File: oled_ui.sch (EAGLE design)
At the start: 30 parts

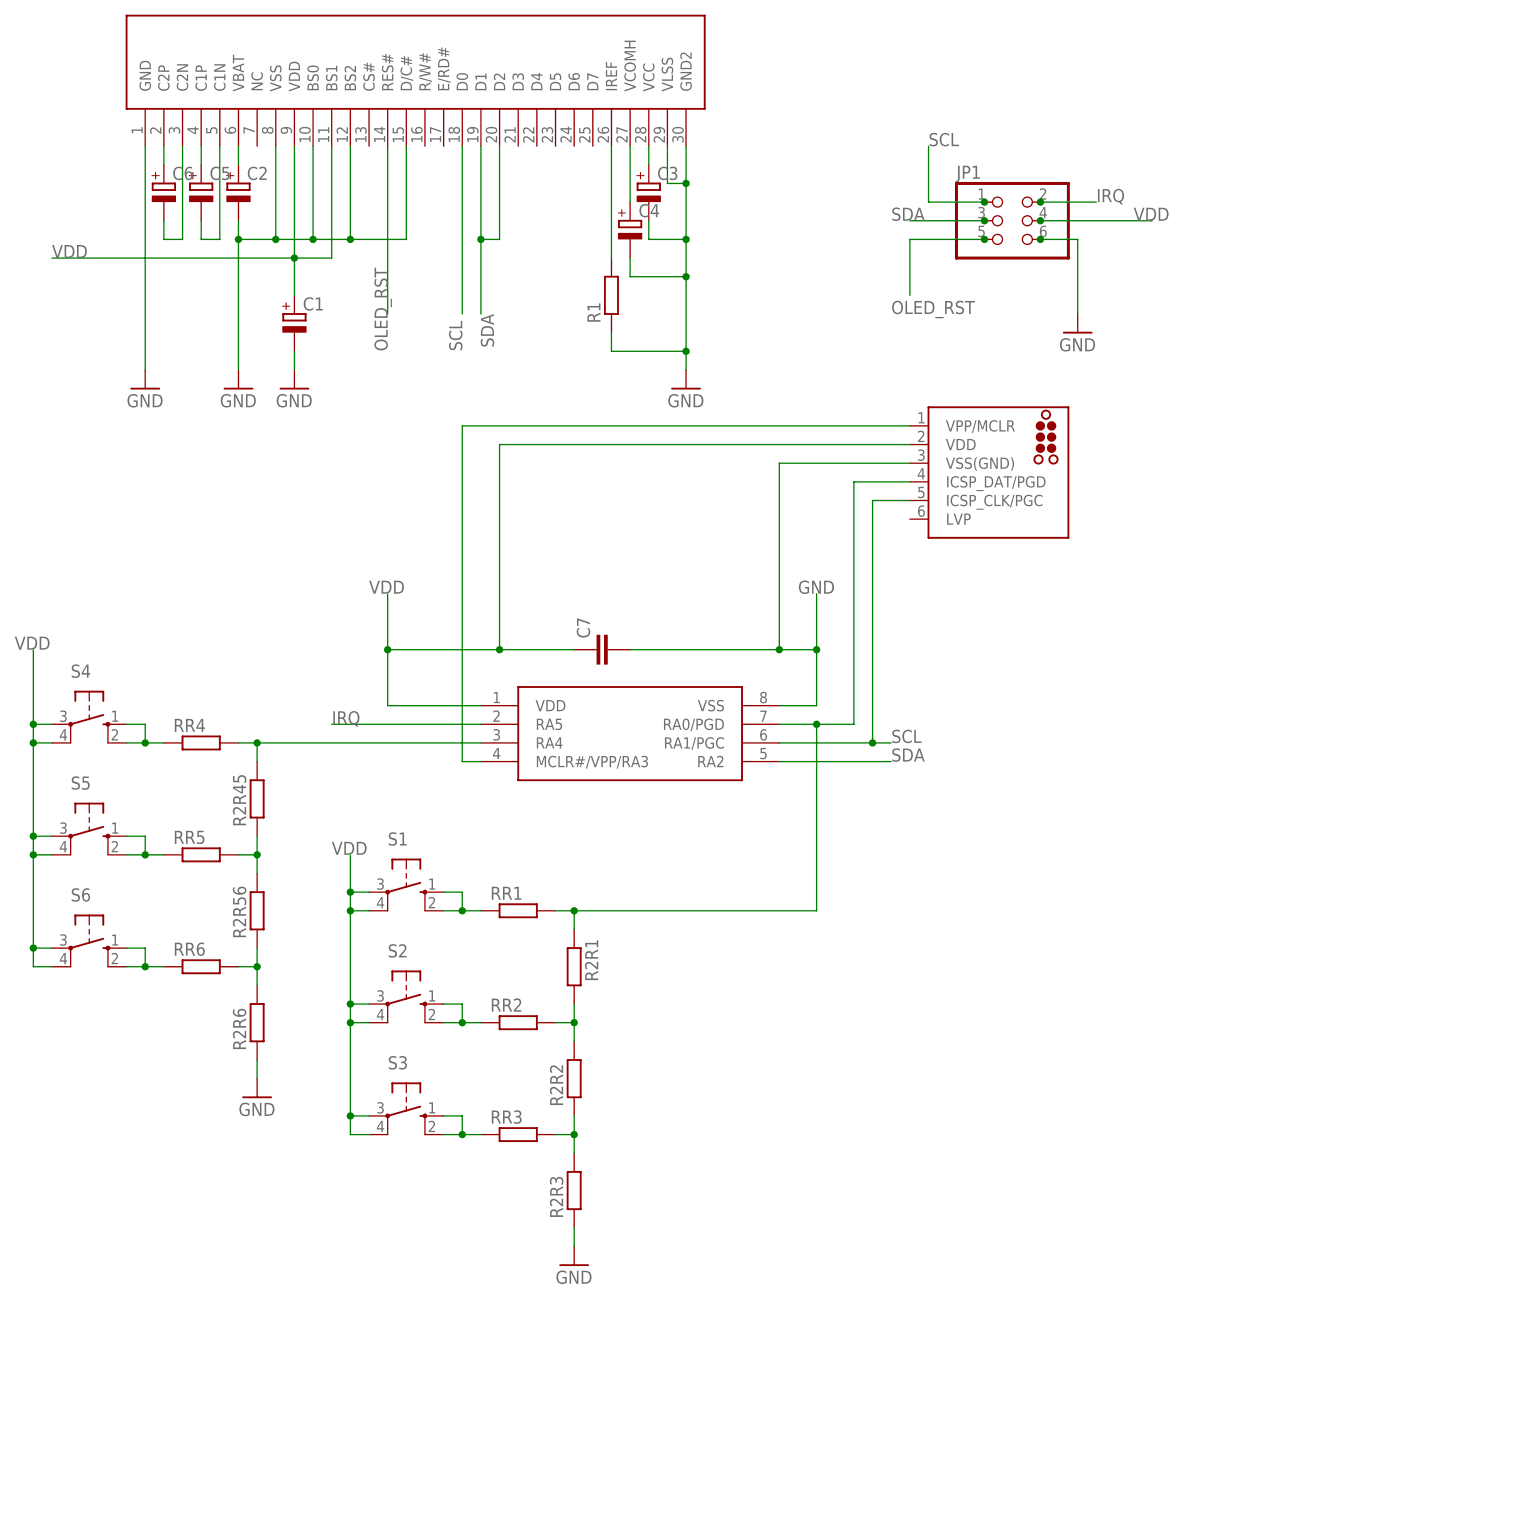
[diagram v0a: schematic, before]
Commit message: updates
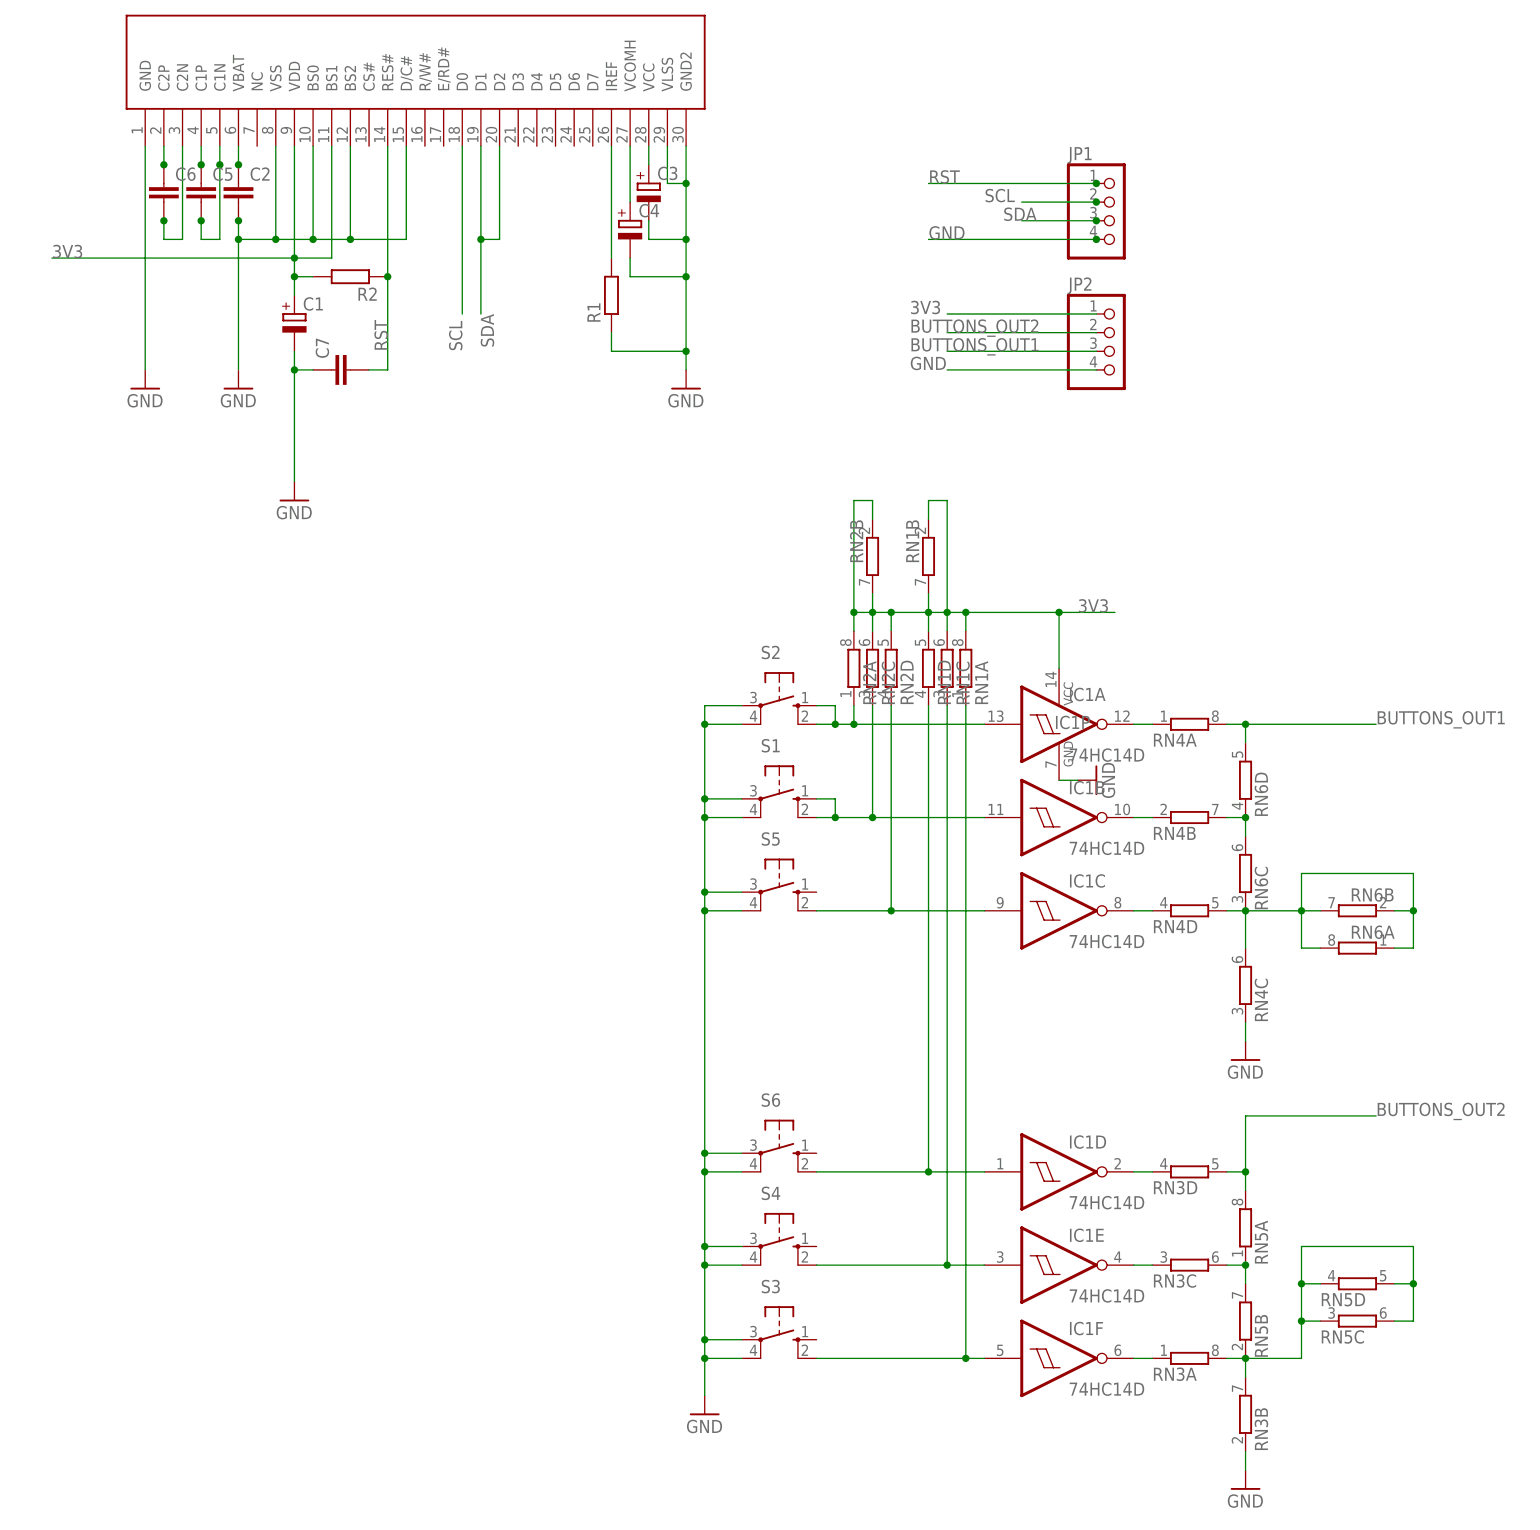
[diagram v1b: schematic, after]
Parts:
- removed J1: (no value), tag-connect:TC2030-MCP-NL
- removed R2R1, R2R2, R2R3, R2R45, R2R56, R2R6, RR1, RR2, RR3, RR4, RR5, RR6: (no value), rcl:R-EU_R0805
- removed U$2: PIC12F1822SO08, jasons_stuff:PIC12F1822SO08
- added IC1: 74HC14D, 74xx-eu:74HC14D
- added JP2: (no value), pinhead:PINHD-1X4
- added R2: (no value), rcl:R-EU_R0805
- added RN1, RN2, RN3, RN4, RN5, RN6: (no value), resistor-dil:4R-NCAY16
- C2, C5, C6: device resistor:CPOL-EUSMCA -> rcl:C-EUC0805
- JP1: device pinhead:PINHD-2X3 -> pinhead:PINHD-1X4
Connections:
- removed net IRQ: JP1.2, U$2.RA5
- removed net OLED_RST: JP1.5, U$1.RES#
- removed net VDD: C1.+, C7.1, J1.VDD, JP1.4, S1.P, S1.P1, S2.P, S2.P1, S3.P, S3.P1, S4.P, S4.P1, S5.P, S5.P1, S6.P, S6.P1, U$1.BS1, U$1.VDD, U$2.VDD
- new net 3V3: C1.+, IC1P.VCC, JP2.1, R2.2, RN1A.2, RN1B.1, RN1B.2, RN1C.2, RN1D.2, RN2A.2, RN2B.1, RN2B.2, RN2C.2, RN2D.2, U$1.BS1, U$1.VDD
- new net BUTTONS_OUT1: JP2.3, RN4A.2, RN6D.2
- new net BUTTONS_OUT2: JP2.2, RN3D.2, RN5A.2
- new net N$22: RN4C.2, RN4D.2, RN6A.1, RN6A.2, RN6B.1, RN6B.2, RN6C.1
- new net N$23: RN3C.2, RN5A.1, RN5B.2
- new net N$26: RN3A.2, RN3B.2, RN5B.1, RN5C.1, RN5C.2, RN5D.1, RN5D.2
- new net RST: C7.2, JP1.1, R2.1, U$1.RES#
- net GND: now also C2.2, C7.1, IC1P.GND, JP1.4, JP2.4, RN3B.1, RN4C.1, S1.P, S1.P1, S2.P, S2.P1, S3.P, S3.P1, S4.P, S4.P1, S5.P, S5.P1, S6.P, S6.P1; no longer C2.-, C7.2, J1.VSS(GND), JP1.6, R2R3.1, R2R6.1, U$2.VSS
- net N$1: now also C6.2; no longer C6.-
- net N$11: now also IC1D.I, RN1D.1, S6.S1; no longer RR1.1, S1.S, S1.S1
- net N$12: now also IC1C.I, RN2D.1, S5.S1; no longer R2R45.2, RR4.2, U$2.RA4
- net N$13: now also IC1B.I, RN2C.1, S1.S, S1.S1; no longer RR2.1, S2.S, S2.S1
- net N$14: now also IC1A.I, RN2A.1, S2.S, S2.S1; no longer RR6.1, S6.S, S6.S1
- net N$15: now also IC1A.O, RN4A.1; no longer RR5.1, S5.S, S5.S1
- net N$16: now also IC1B.O, RN4B.1; no longer RR4.1, S4.S, S4.S1
- net N$17: now also IC1C.O, RN4D.1; no longer RR3.1, S3.S, S3.S1
- net N$18: now also IC1E.O, RN3C.1; no longer J1.ICSP_DAT/PGD, R2R1.1, RR1.2, U$2.RA0/PGD
- net N$19: now also IC1D.O, RN3D.1; no longer R2R1.2, R2R2.2, RR2.2
- net N$2: now also C6.1; no longer C6.+
- net N$20: now also IC1F.O, RN3A.1; no longer R2R2.1, R2R3.2, RR3.2
- net N$21: now also RN4B.2, RN6C.2, RN6D.1; no longer J1.VPP/MCLR, U$2.MCLR#/VPP/RA3
- net N$3: now also C5.1; no longer C5.+
- net N$4: now also C5.2; no longer C5.-
- net N$5: now also IC1F.I, RN1A.1, S3.S1; no longer R2R56.1, R2R6.2, RR6.2
- net N$7: now also C2.1; no longer C2.+
- net N$9: now also IC1E.I, RN1C.1, S4.S1; no longer R2R45.1, R2R56.2, RR5.2
- net SCL: now also JP1.2; no longer J1.ICSP_CLK/PGC, JP1.1, U$2.RA1/PGC
- net SDA: no longer U$2.RA2
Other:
- moved on the sheet: C7, S1, S2, S3, S4, S5, S6
